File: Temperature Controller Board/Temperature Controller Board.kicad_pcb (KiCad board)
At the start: 2 copper layers, 46.9 x 55.4 mm, 18 parts, among them J2 Pwr, J4 AC Line, J5 Rotary Encoder Board, J6 LEDS, K1 G3MB-202PDC5 Relay, U1 AZ1117-5.0

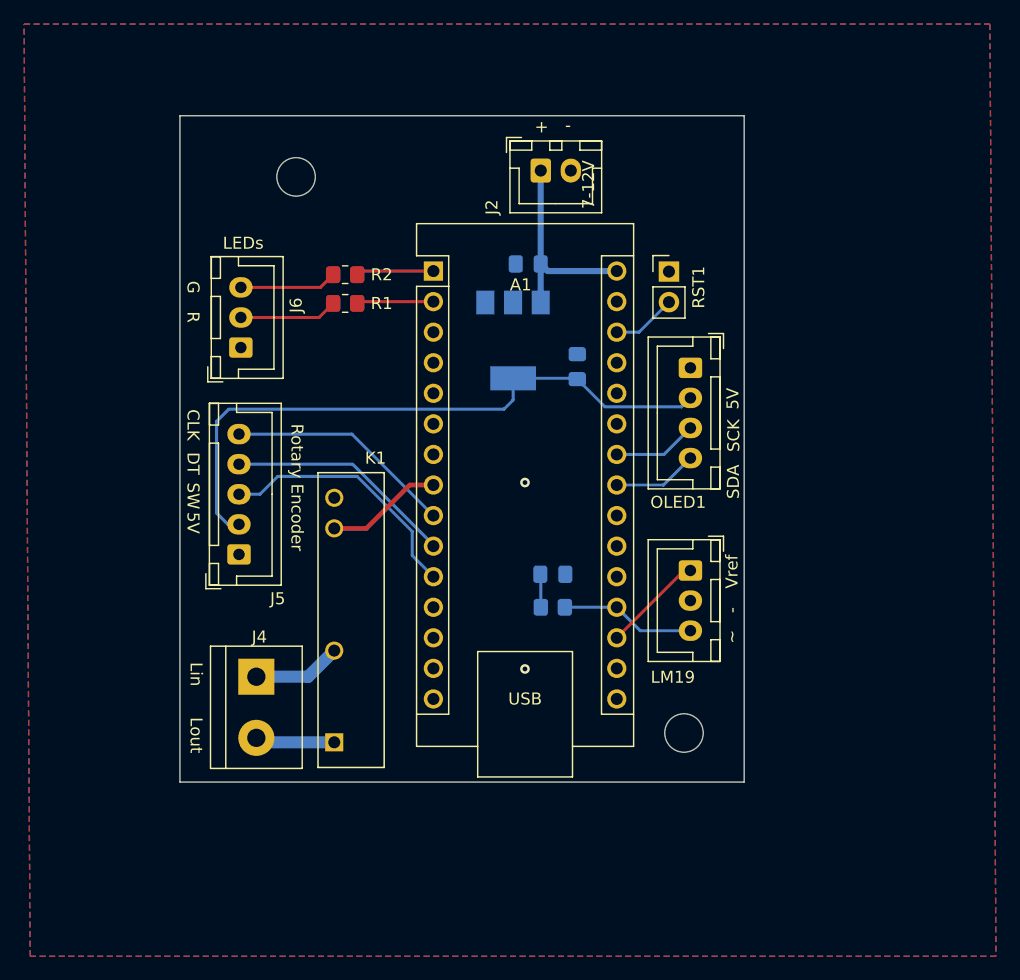
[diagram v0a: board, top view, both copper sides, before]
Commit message: updated Schematic and PCB
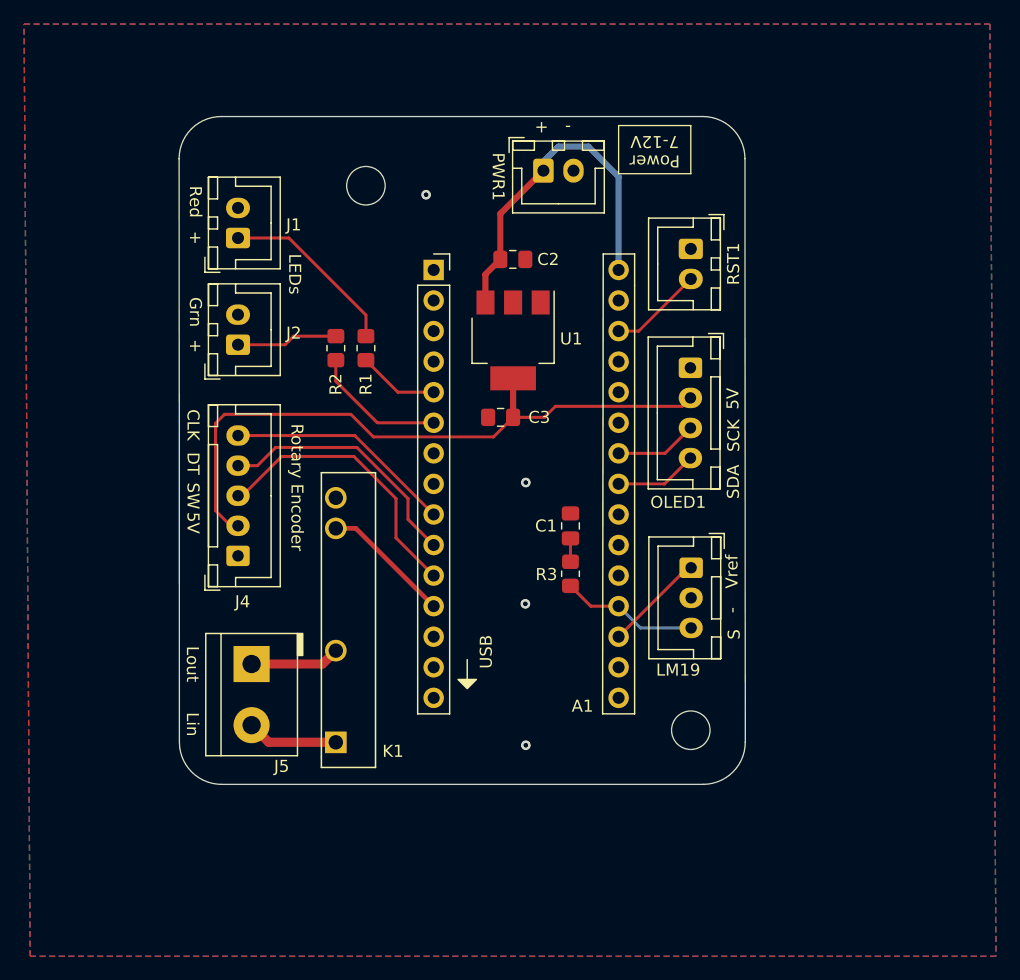
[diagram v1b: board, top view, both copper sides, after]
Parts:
- removed J6: LEDS, Connector_JST:JST_XH_B3B-XH-A_1x03_P2.50mm_Vertical
- removed LM1: LM19, Connector_JST:JST_XH_B3B-XH-A_1x03_P2.50mm_Vertical
- added J1: Conn_01x02, Connector_JST:JST_XH_B2B-XH-A_1x02_P2.50mm_Vertical, F.Cu at (102.9, 69.6)
- added LM19: LM19, Connector_JST:JST_XH_B3B-XH-A_1x03_P2.50mm_Vertical, F.Cu at (140.5, 97.0)
- added PWR1: Conn_01x02, Connector_JST:JST_XH_B2B-XH-A_1x02_P2.50mm_Vertical, F.Cu at (128.2, 64.0)
- A1: footprint Module:Arduino_Nano -> 000_Thomas_Footprints:Arduino Riser
- C1, C2, C3, R3, U1: moved to F.Cu
- J2: value Pwr -> Conn_01x02
- J4: value AC Line -> Conn_01x05; footprint TerminalBlock:TerminalBlock_bornier-2_P5.08mm -> Connector_JST:JST_XH_B5B-XH-A_1x05_P2.50mm_Vertical
- J5: value Rotary Encoder Board -> Conn_01x02; footprint Connector_JST:JST_XH_B5B-XH-A_1x05_P2.50mm_Vertical -> 000_Thomas_Footprints:myTerminalBlock-2_P5.08mm
- K1: value G3MB-202PDC5 Relay -> AQG22105; footprint 000_Thomas_Footprints:G3MB-202PDC5 Relay -> 000_Thomas_Footprints:RELAY_AQG22105
- OLED1: value ~ -> Conn_01x04
- RST1: value RST Button -> Conn_01x02; footprint Connector_PinHeader_2.54mm:PinHeader_1x02_P2.54mm_Vertical -> Connector_JST:JST_XH_B2B-XH-A_1x02_P2.50mm_Vertical
- moved J2 29.0 mm to (102.9, 78.5), turned to 90 degrees
- moved A1 19.8 mm to (126.9, 90.5)
- moved J5 11.6 mm to (105.0, 107.3), turned to -90 degrees
- moved J4 10.2 mm to (102.9, 96.0), turned to 90 degrees
- moved C3 7.64 mm to (124.7, 84.5), turned to 180 degrees
- moved R2 6.16 mm to (111.0, 78.8), turned to -90 degrees
- moved H1 5.85 mm to (113.5, 65.2)
- moved C1 4.27 mm to (130.5, 93.5), turned to -90 degrees
- moved R1 4.10 mm to (113.5, 78.8), turned to -90 degrees
- moved R3 3.15 mm to (130.5, 97.5), turned to -90 degrees
- moved RST1 2.62 mm to (140.5, 70.5), turned to -90 degrees
- moved K1 1.97 mm to (112.0, 101.3)
- moved C2 1.34 mm to (125.7, 71.4), turned to 0 degrees
- moved H2 0.61 mm to (140.5, 110.5)
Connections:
- A1 pad 1: /RED_PIN -> unconnected-(A1-D1/TX-Pad1)
- A1 pad 12: unconnected-(A1-D9-Pad12) -> /relay
- A1 pad 18: /Aref -> /Vref
- A1 pad 2: /GREEN_PIN -> unconnected-(A1-D0/RX-Pad2)
- A1 pad 5: unconnected-(A1-D2-Pad5) -> /RED_PIN
- A1 pad 6: unconnected-(A1-D3-Pad6) -> /GREEN_PIN
- A1 pad 8: /relay -> unconnected-(A1-D5-Pad8)
- J2 pad 1: /Vin -> /GREEN_LED
- J4 pad 1: Net-(J4-Pin_1) -> GND
- J4 pad 2: Net-(J4-Pin_2) -> /5V
- J5 pad 1: GND -> Net-(J5-Pin_1)
- J5 pad 2: /5V -> Net-(J5-Pin_2)
- K1 pad 1: Net-(J4-Pin_2) -> Net-(J5-Pin_2)
- K1 pad 2: Net-(J4-Pin_1) -> Net-(J5-Pin_1)
- R1 pad 1: /GREEN_LED -> /RED_LED
- R1 pad 2: /GREEN_PIN -> /RED_PIN
- R2 pad 1: /RED_LED -> /GREEN_LED
- R2 pad 2: /RED_PIN -> /GREEN_PIN
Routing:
- net /Vin: track 17.6 -> 29.3 mm
- net /Aref: track 8.44 -> 0.00 mm
- net /Vref: track 0.00 -> 8.40 mm
- net Net-(J5-Pin_2): track 0.00 -> 7.59 mm
- net Net-(J5-Pin_1): track 0.00 -> 7.46 mm
- net Net-(J4-Pin_1): track 7.37 -> 0.00 mm
- net /RED_LED: track 8.11 -> 15.0 mm
- net Net-(J4-Pin_2): track 6.63 -> 0.00 mm
- net /GREEN_PIN: track 6.39 -> 11.3 mm
- net /RST: track 5.37 -> 7.79 mm
- net /SWT_en: track 21.4 -> 23.6 mm
- net /DT_en: track 19.0 -> 21.3 mm
- net /5V: track 53.1 -> 54.8 mm
- net /relay: track 9.73 -> 10.8 mm
- net Net-(C1-Pad2): track 2.76 -> 1.94 mm
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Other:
- board size 46.9 x 55.4 mm -> 47.1 x 55.5 mm
- board text added: "Grn"
- board text added: "Power 7-12V"
- board text added: "Red"
- board text added: "S"
- board text added: "UVic AMO Lab PID Temperature Controller Designed by: Thomas Bourgeois"
- board text removed: "7-12V"
- board text removed: "G"
- board text removed: "LM19"
- board text removed: "R"
- board text removed: "~"
